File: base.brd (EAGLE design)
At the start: 53.3 x 29.2 mm, 16 parts

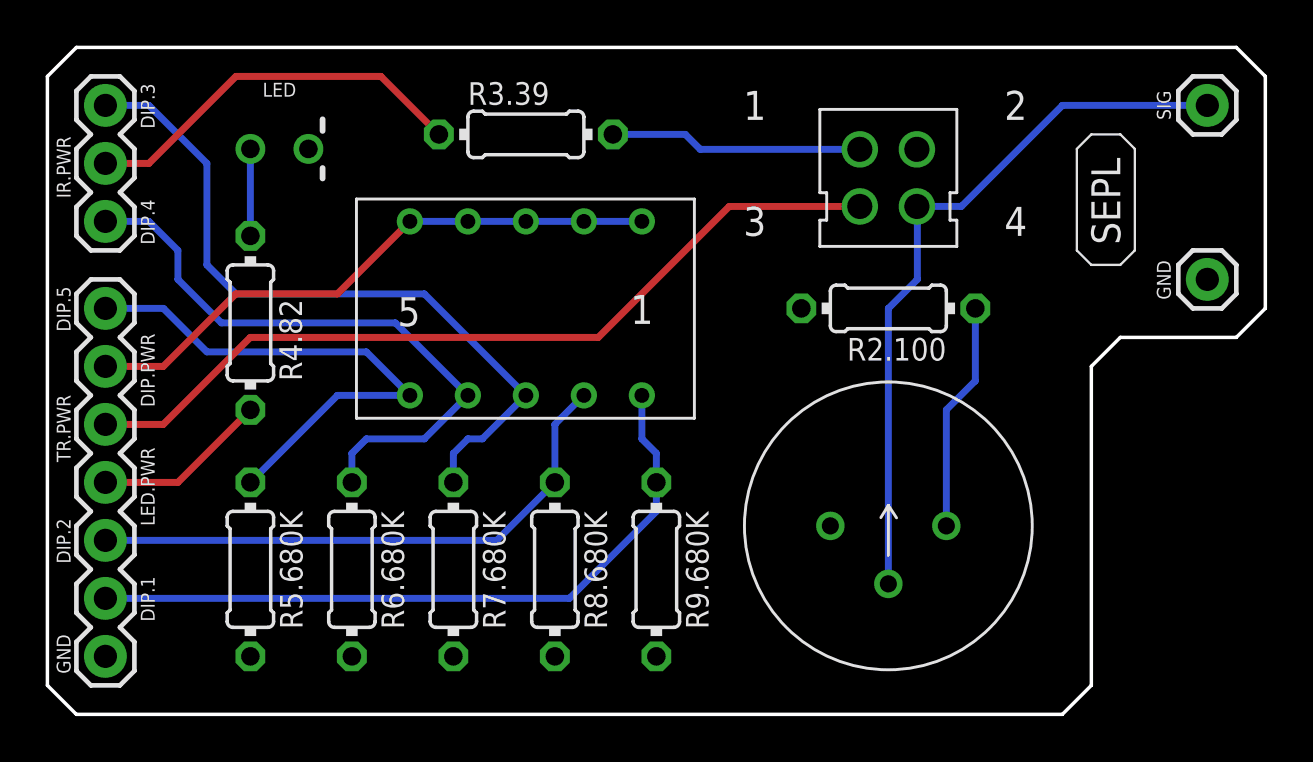
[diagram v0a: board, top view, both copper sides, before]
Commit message: updated layout and part
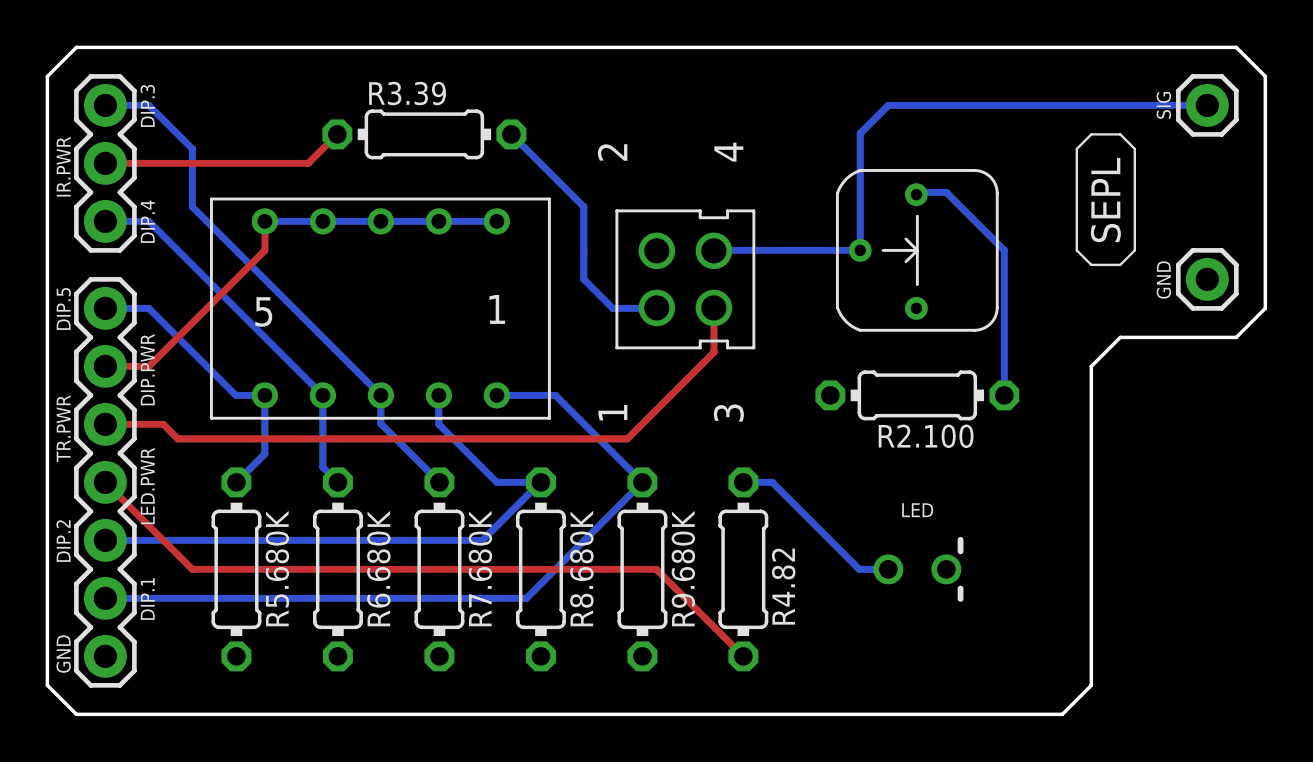
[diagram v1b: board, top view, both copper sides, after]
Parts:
- removed R1.10K: 93PR10KLF, ferraris_sensor_project:93PR10KLF
- added U$3: CT6EP103, ferraris_sensor_project:CT6EP103
- moved LED 33.5 mm to (63.5, 39.4)
- moved R4.82 24.1 mm to (55.9, 39.4)
- moved U$1 9.94 mm to (53.3, 52.1), turned to 90 degrees
- moved U$2 6.35 mm to (45.1, 47.0)
- moved R3.39 4.45 mm to (41.9, 58.4)
- moved R2.100 4.02 mm to (63.5, 47.0)
- moved R5.680K 0.61 mm to (33.7, 39.4)
- moved R6.680K 0.61 mm to (38.1, 39.4)
- moved R7.680K 0.61 mm to (42.6, 39.4)
- moved R8.680K 0.61 mm to (47.0, 39.4)
- moved R9.680K 0.61 mm to (51.5, 39.4)
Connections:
- net N$1: now also U$3.1; no longer R1.10K.1
- net P$1: now also U$3.3; no longer R1.10K.3
- net SIG: now also U$3.2; no longer R1.10K.2
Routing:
- net LED_PWR: track 7.67 -> 31.1 mm
- net DIP_5: track 23.5 -> 12.9 mm
- net DIP_4: track 27.2 -> 16.8 mm
- net DIP_3: track 31.8 -> 23.7 mm
- net TR_PWR: track 37.0 -> 30.4 mm
- net IR_PWR: track 17.2 -> 10.7 mm
- net DIP_PWR: track 26.1 -> 20.5 mm
- net SIG: track 31.6 -> 27.2 mm
- net N$3: track 3.81 -> 7.93 mm
- net DIP_1: track 31.1 -> 33.6 mm
- net DIP_2: track 25.1 -> 26.9 mm
- net N$1: track 10.1 -> 11.3 mm
